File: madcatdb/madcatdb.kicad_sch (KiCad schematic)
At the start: 9 parts, among them J1 Conn_01x04

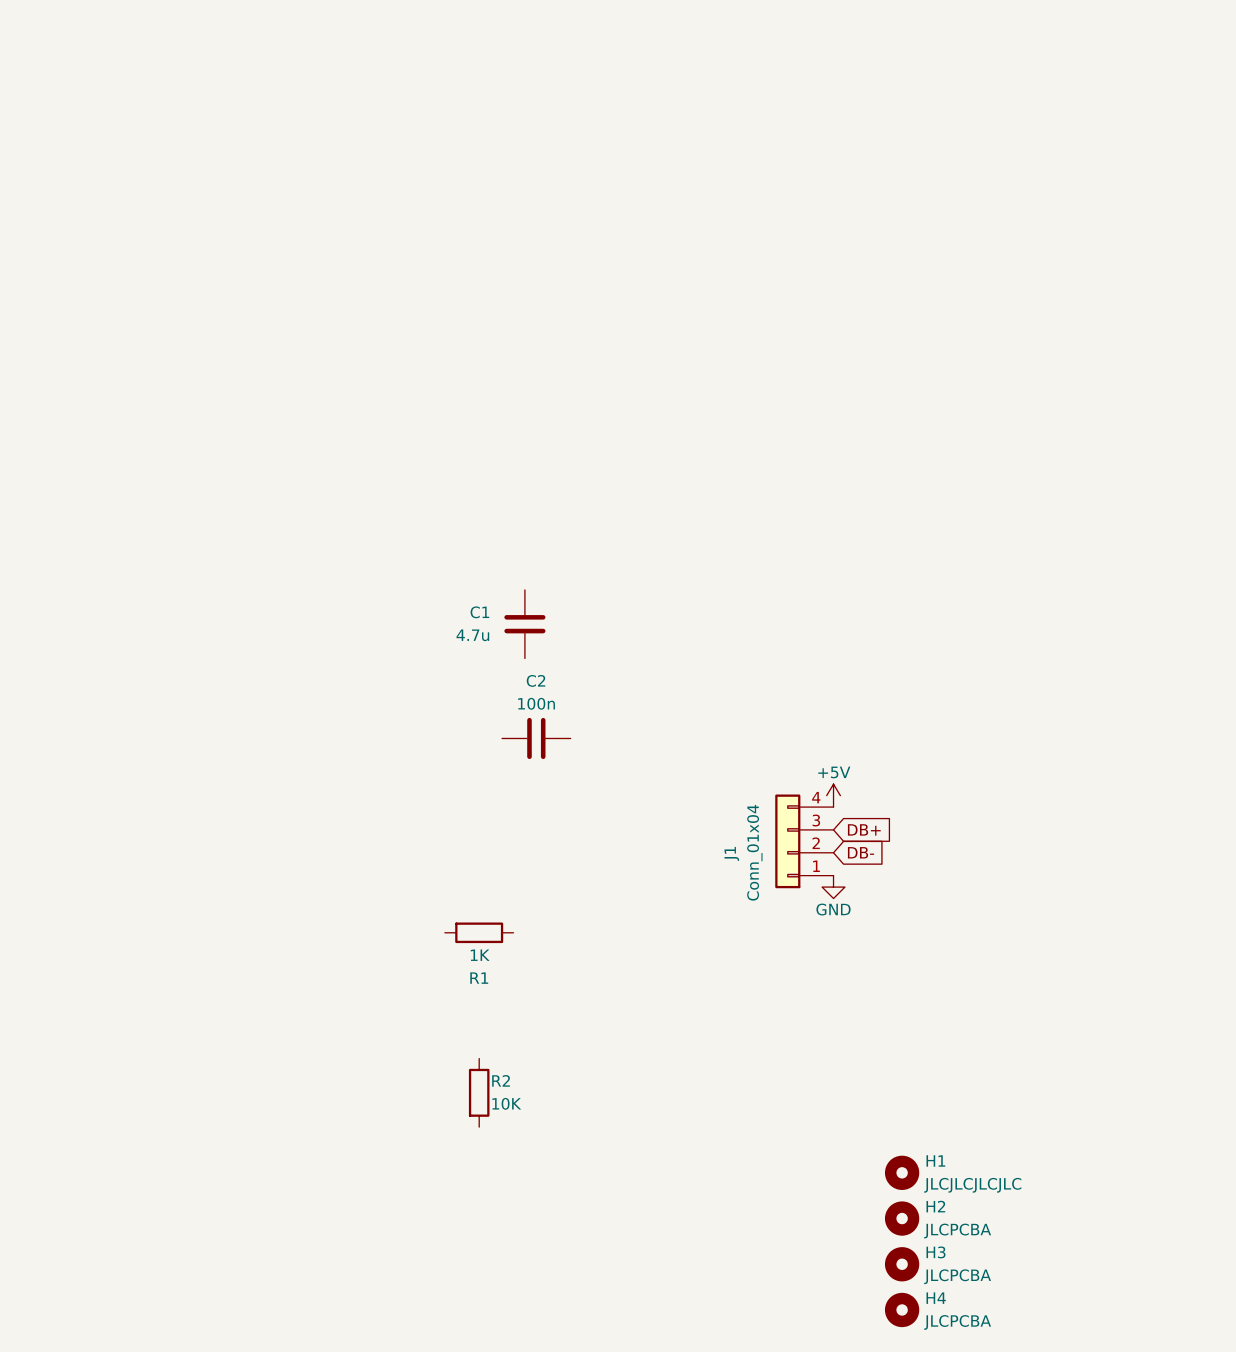
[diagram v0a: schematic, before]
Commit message: done (lol)
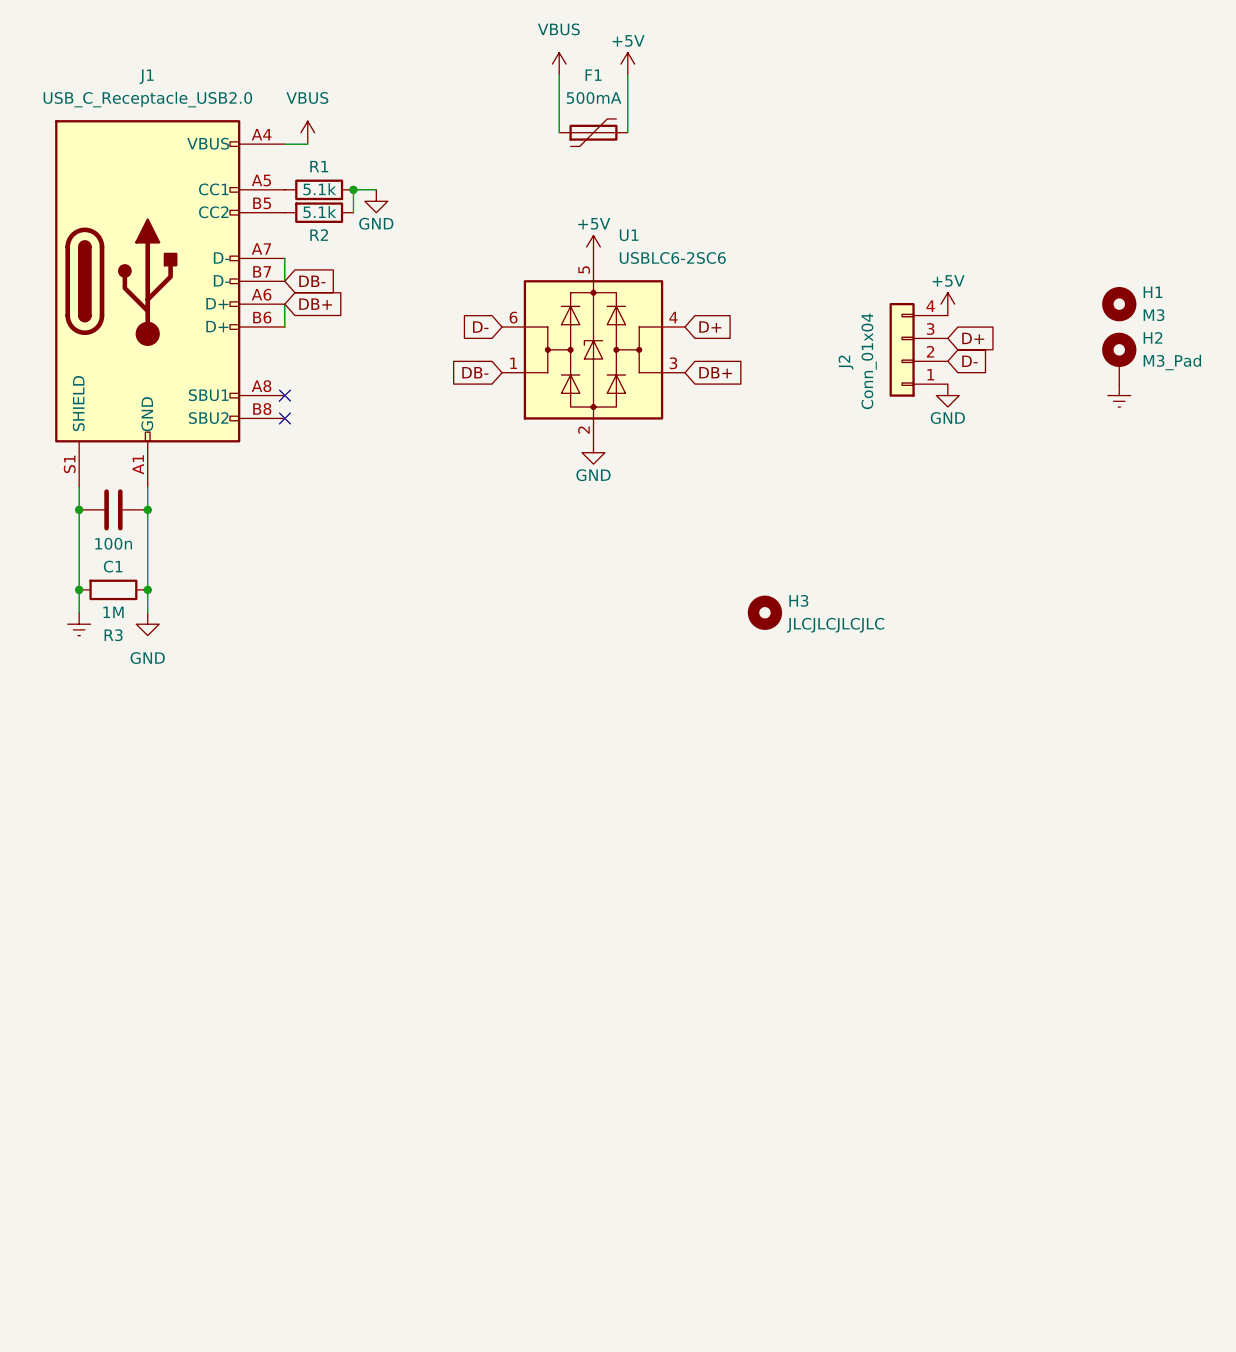
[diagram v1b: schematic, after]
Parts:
- removed C1: 4.7u, Crokto:C_0603_1608Metric, symbol Device:C
- removed H2, H3, H4: JLCPCBA, Crokto:JLCPCBA, symbol Mechanical:MountingHole
- added F1: 500mA, Fuse:Fuse_1206_3216Metric, symbol Device:Polyfuse
- added H1: M3, Crokto:M3_Via_Hole_NC, symbol Mechanical:MountingHole
- added H2: M3_Pad, Crokto:M3_Via_Hole, symbol Mechanical:MountingHole_Pad
- added J1: USB_C_Receptacle_USB2.0, Crokto:USB_C_Receptacle_HRO_TYPE-C-31-M-12, symbol Connector:USB_C_Receptacle_USB2.0
- added R3: 1M, Resistor_SMD:R_1206_3216Metric, symbol Device:R
- added U1: USBLC6-2SC6, Package_TO_SOT_SMD:SOT-23-6, symbol Power_Protection:USBLC6-2SC6
- C1: renamed from C2; footprint Crokto:C_0603_1608Metric -> Capacitor_SMD:C_1206_3216Metric; LCSC C14663 -> (none)
- J2: renamed from J1; LCSC C160404 -> (none)
- R1: value 1K -> 5.1k; LCSC C21190 -> (none)
- R2: value 10K -> 5.1k; LCSC C25804 -> (none)
- renumbered H1 to H3
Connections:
- net +5V: now also F1.2, U1.5 (VBUS)
- net DB+: now also J1.A6 (D+), J1.B6 (D+), U1.3 (I/O2); no longer J2.3 (Pin_3)
- net DB-: now also J1.A7 (D-), J1.B7 (D-), U1.1 (I/O1); no longer J2.2 (Pin_2)
- net GND: now also C1.1, R1.2, R2.1, J1.A1 (GND), J1.A12 (GND), J1.B1 (GND), J1.B12 (GND), R3.1, U1.2 (GND)
- net Earth: now reaches C1.2
- net Earth: now also H2.1, J1.S1 (SHIELD), R3.2
- net at R1.1: now also J1.A5 (CC1)
- net at R2.2: now also J1.B5 (CC2)
- new net D+: J2.3 (Pin_3), U1.4 (I/O2)
- new net D-: J2.2 (Pin_2), U1.6 (I/O1)
- new net VBUS: F1.1, J1.A4 (VBUS), J1.A9 (VBUS), J1.B4 (VBUS), J1.B9 (VBUS)
- no-connect marks 0 -> 2
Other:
- moved on the sheet: C1, H3, J2, R1
